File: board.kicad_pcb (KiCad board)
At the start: 2 copper layers, 96.3 x 46.3 mm, 38 parts, among them J0 Battery Pads, J1 PGRM, J2 Micro SD Slot, J3 USB_B_Micro, SW0 RESET, SW1 UP, SW2 DOWN, SW3 LEFT, SW4 RIGHT, SW5 BTN_A, SW6 BTN_B, SW7 BTN_C, SW8 POWER, U0 ATmega1284P, U1 OLED, U2 CHG, U3 Reg, Y1 16MHz

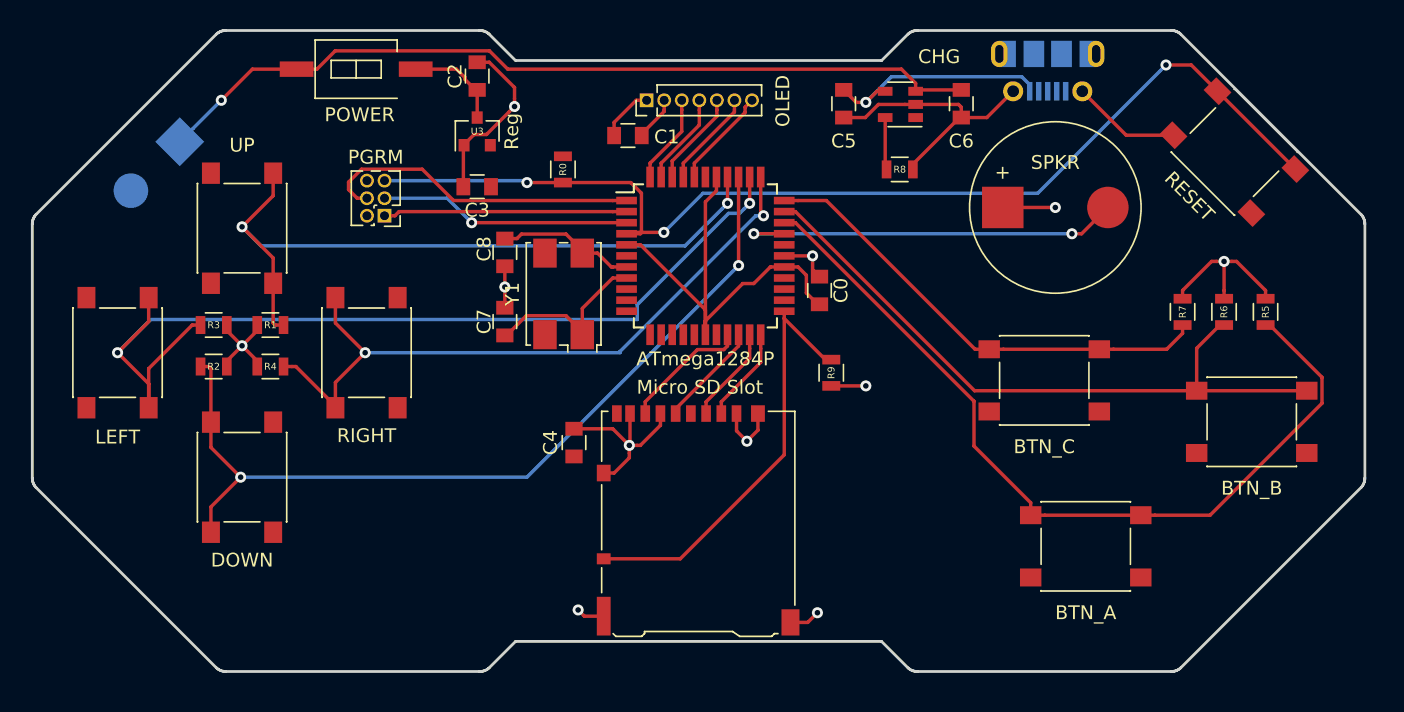
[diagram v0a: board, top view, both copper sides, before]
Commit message: Revert "added crystal"
This reverts commit 60f505991b0e3ccfce5c63fb45a6584053ac2d9c.
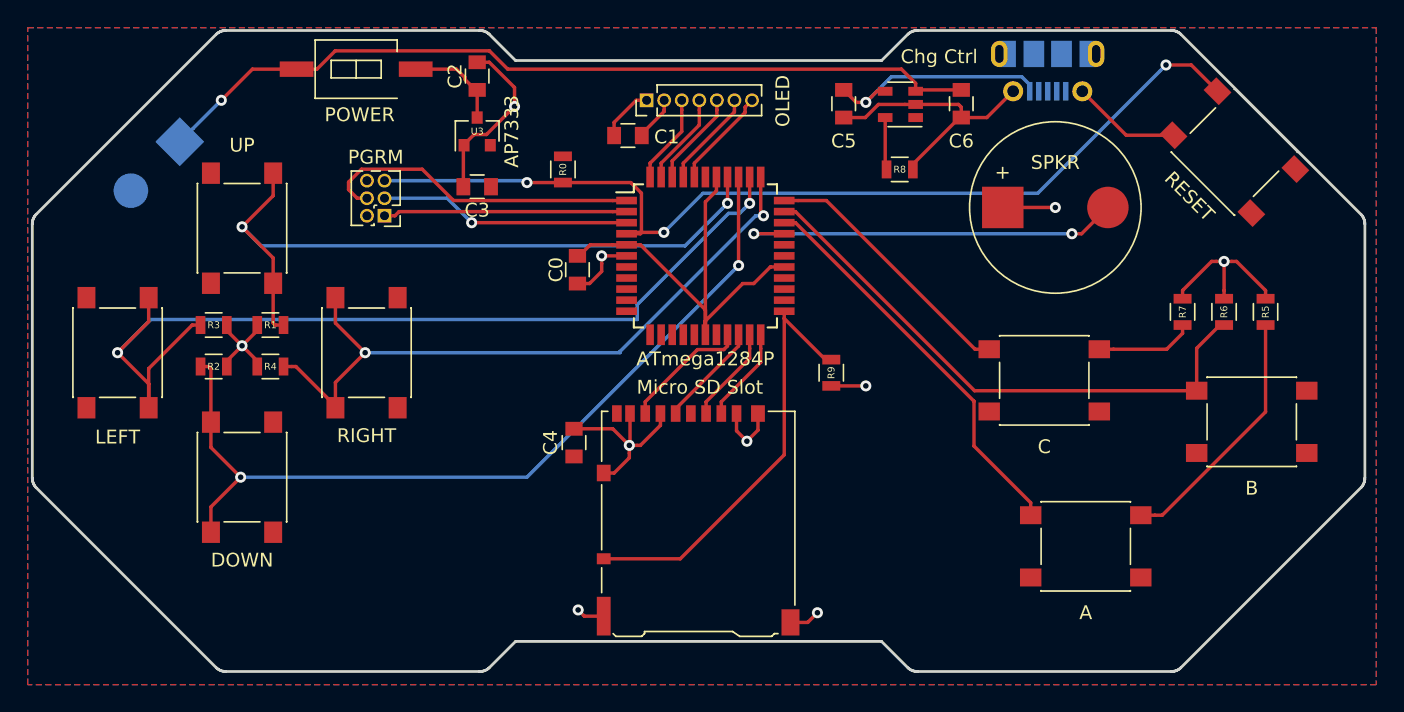
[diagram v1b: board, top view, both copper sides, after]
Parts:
- removed C7, C8: 22pF, Capacitors_SMD:C_0805
- removed Y1: 16MHz, Crystals:Crystal_SMD_7050-4pin_7.0x5.0mm
- SW5: value BTN_A -> A
- SW6: value BTN_B -> B
- SW7: value BTN_C -> C
- U2: value CHG -> Chg Ctrl
- U3: value Reg -> AP7333
- moved C0 17.6 mm to (142.2, 100.0), turned to 270 degrees
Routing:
- net BTN_A: track 60.9 -> 47.4 mm
- net Net-(U0-Pad8): track 12.9 -> 0.00 mm
- net Net-(U0-Pad7): track 10.0 -> 0.00 mm
- net RESET: track 79.4 -> 71.5 mm
- net BTN_C: track 34.3 -> 26.4 mm
- net BTN_B: track 48.9 -> 40.9 mm
- net GND: track 99.3 -> 97.5 mm, vias 11 -> 10
- net +3V3: track 37.1 -> 36.6 mm
- added copper zone on F.Cu, net +3V3
- added copper zone on B.Cu, net GND
